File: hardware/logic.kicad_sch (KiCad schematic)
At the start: 10 parts, among them IC1 UCC2946DG4, U13 74HCS08

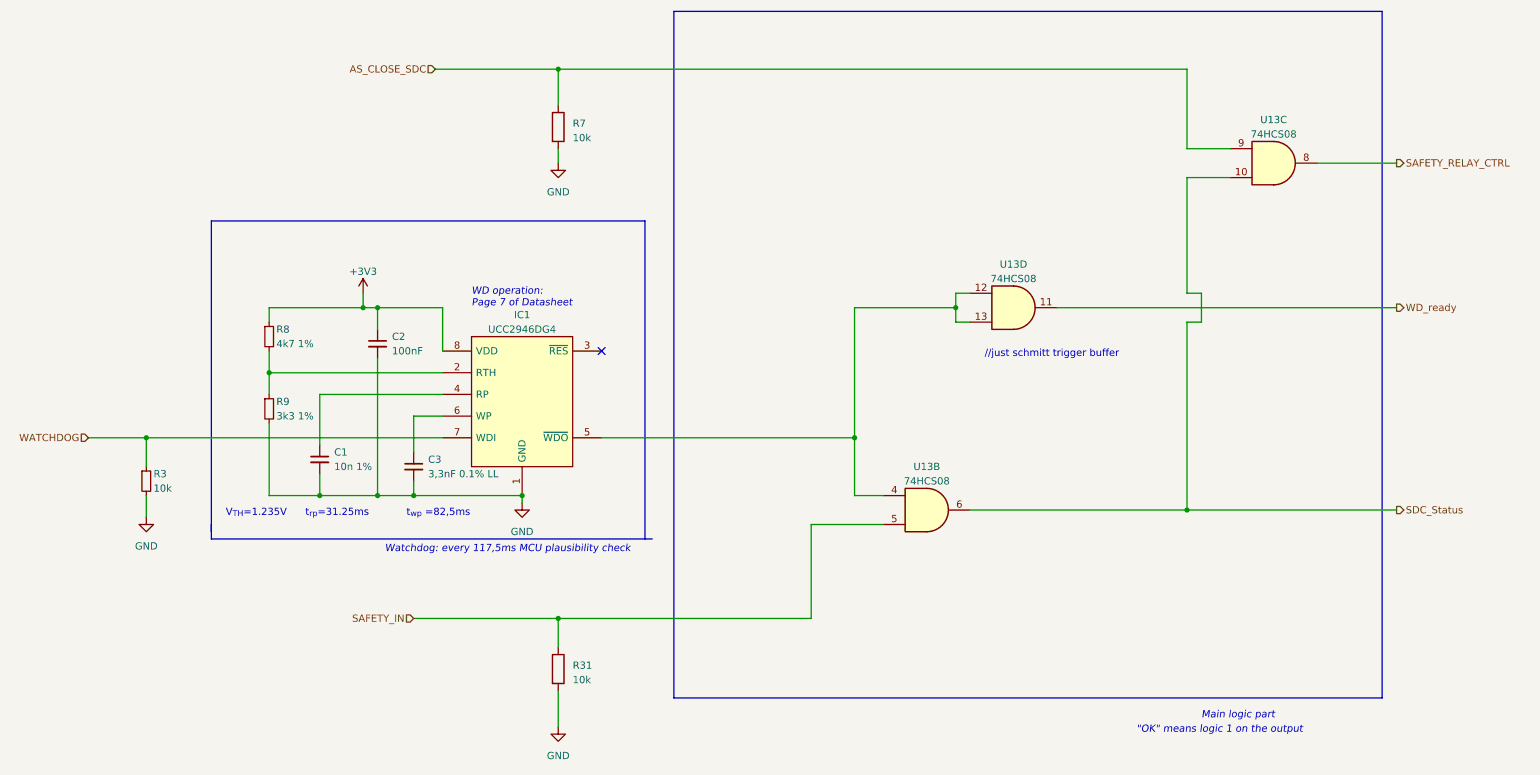
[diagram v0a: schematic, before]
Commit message: WIP revision 2 layout refinement
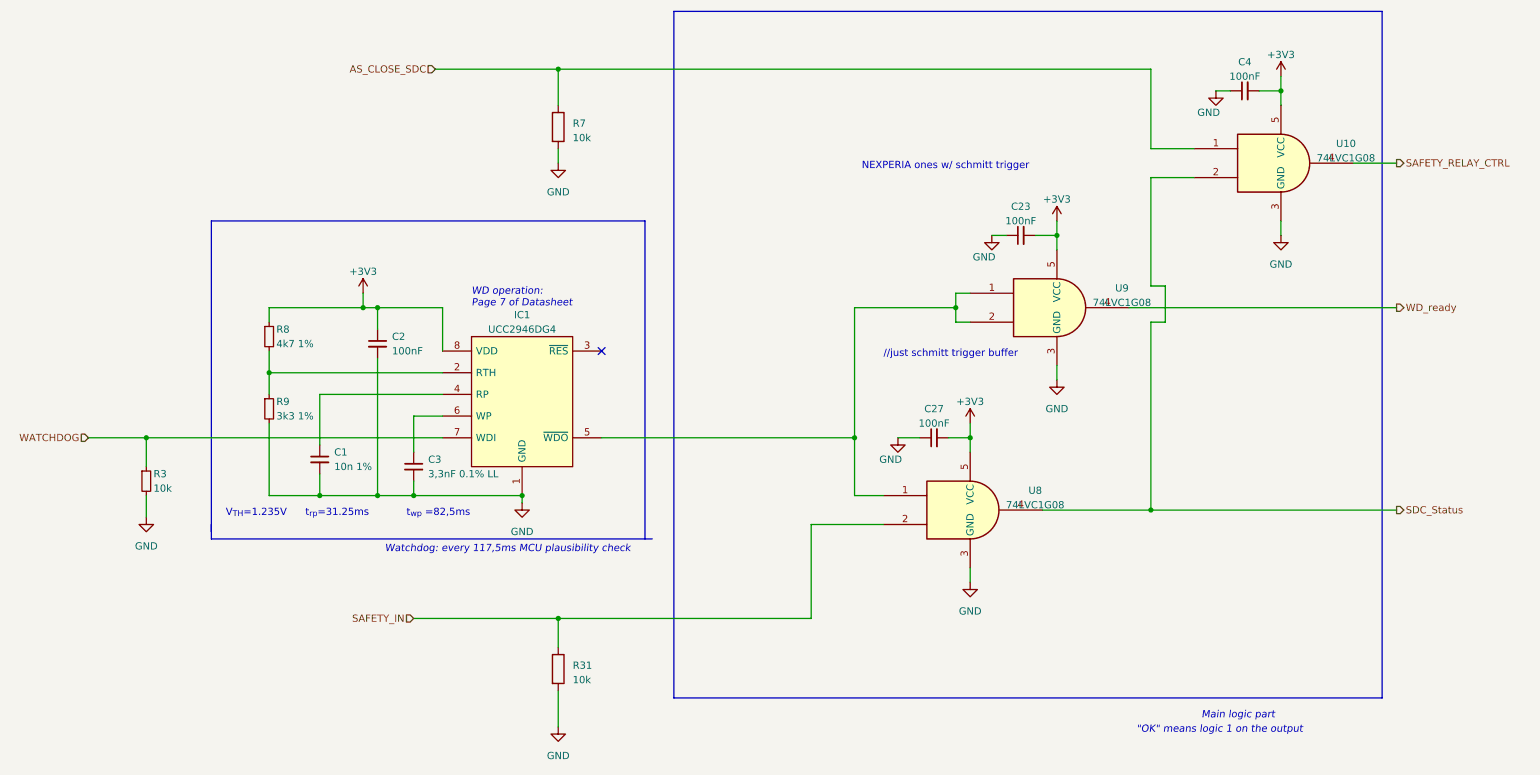
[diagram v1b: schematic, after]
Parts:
- removed U13: 74HCS08, Package_SO:SOIC-14_3.9x8.7mm_P1.27mm, symbol 74xx:74LS08
- added C23, C27, C4: 100nF, Capacitor_SMD:C_0603_1608Metric_Pad1.08x0.95mm_HandSolder, symbol Device:C_Small
- added U10, U8, U9: 74LVC1G08, Package_TO_SOT_SMD:SOT-353_SC-70-5_Handsoldering, symbol 74xGxx:74LVC1G08
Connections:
- net +3V3: now also C23.2, C27.2, C4.2, U10.5 (VCC), U8.5 (VCC), U9.5 (VCC)
- net AS_CLOSE_SDC: now also U10.1
- net GND: now also C23.1, C27.1, C4.1, U10.3 (GND), U8.3 (GND), U9.3 (GND)
- net SAFETY_IN: now also U8.2
- net SAFETY_RELAY_CTRL: now also U10.4
- net SDC_Status: now also U10.2, U8.4
- net WD_ready: now also U9.4
- net at IC1.5 (~{WDO}): now also U8.1, U9.1, U9.2
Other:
- note added: "NEXPERIA ones w/ schmitt trigger"
